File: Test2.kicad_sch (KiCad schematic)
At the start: 14 parts, among them J1 Raspberry_Pi_2_3, J1_GPIO4 01×06, J2_GPIO17 Conn_01x06_Socket, J3_GPIO27 Conn_01x06_Socket, J4_GPIO22 Conn_01x06_Socket, M1_GPIO23 Motor_Servo, SW1_GPIO8 SW_Push

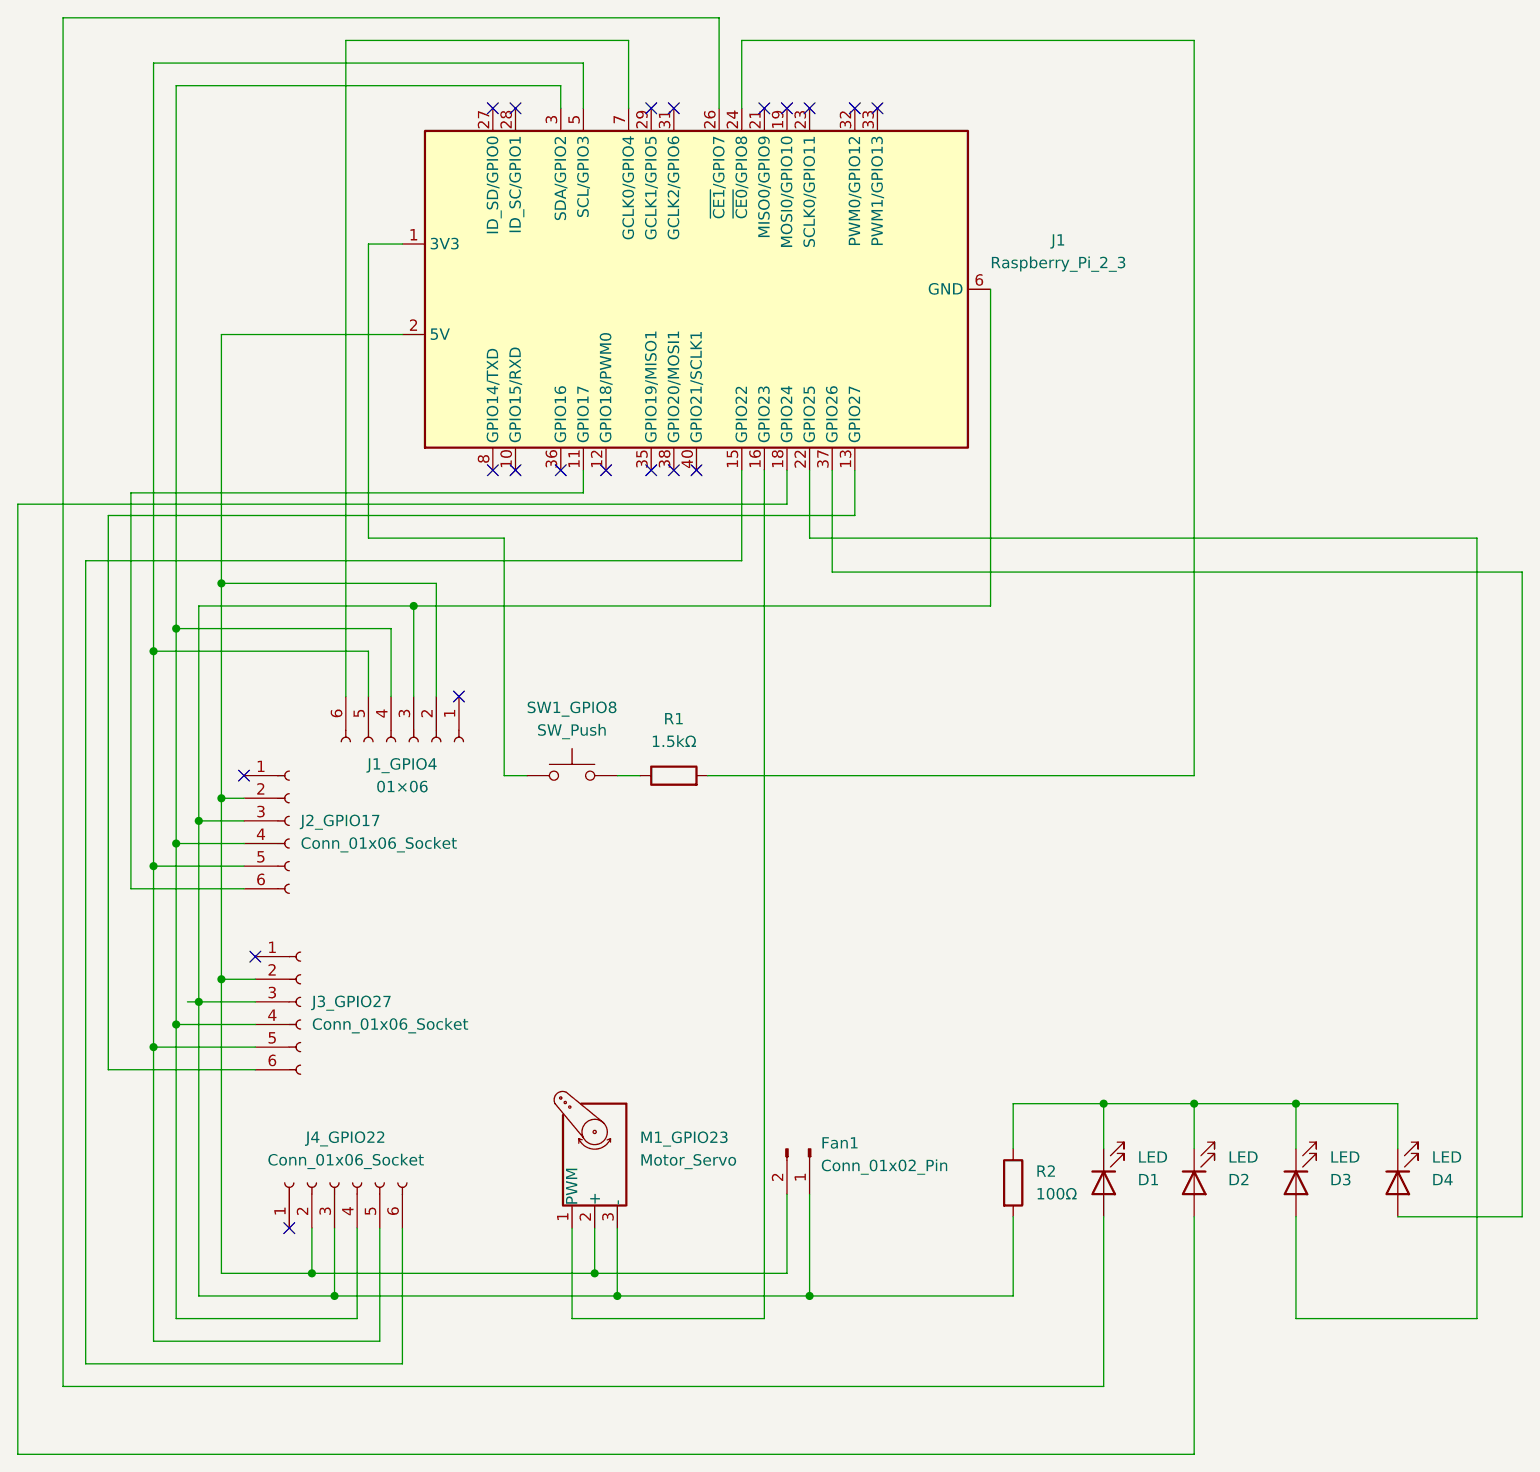
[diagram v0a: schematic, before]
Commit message: Initial commit
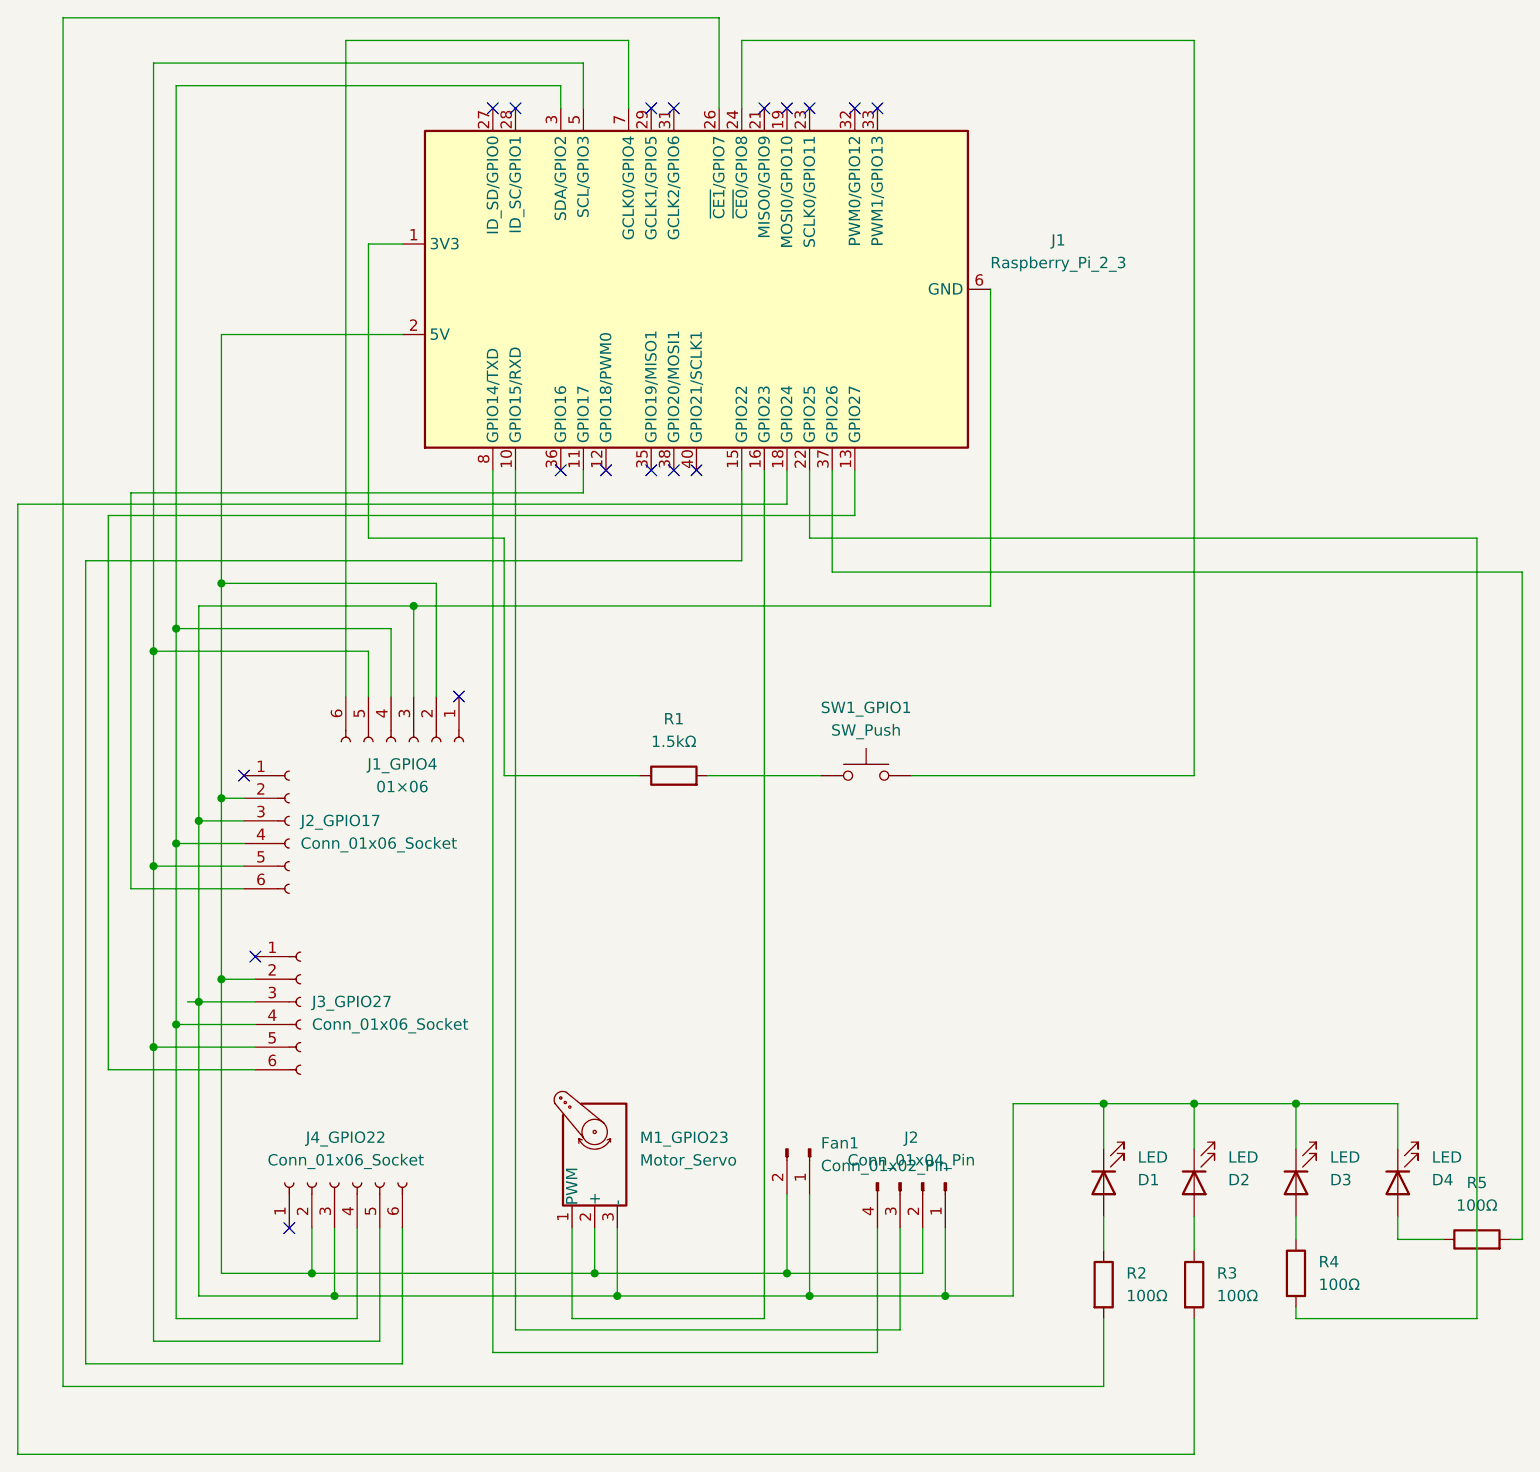
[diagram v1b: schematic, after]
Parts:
- removed SW1_GPIO8: SW_Push, ZHpretty:PushButton, symbol Switch:SW_Push
- added J2: Conn_01x04_Pin, Library:Grove_1x04, symbol Connector:Conn_01x04_Pin
- added R3, R4, R5: 100Ω, Resistor_SMD:R_0805_2012Metric, symbol Device:R
- added SW1_GPIO1: SW_Push, ZHpretty:PushButton, symbol Switch:SW_Push
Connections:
- net at Fan1.2 (Pin_2), J1.2 (5V), J1.4 (5V)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: now also J2.2 (Pin_2)
- net at Fan1.1 (Pin_1), J1.14 (GND), J1.20 (GND)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: now also D1.1 (K), D2.1 (K), D3.1 (K), D4.1 (K), J2.1 (Pin_1); no longer R2.2
- net at D2.2 (A): now also R3.1; no longer J1.18 (GPIO24)
- net at R1.1: now also J1.1 (3V3), J1.17 (3V3)
- net at R1.2: now also SW1_GPIO1.1; no longer J1.24 (~{CE0}/GPIO8)
- net at J1.10 (GPIO15/RXD): now also J2.3 (Pin_3)
- net at J1.22 (GPIO25): now also R4.2; no longer D3.2 (A)
- net at D1.2 (A): now also R2.1; no longer J1.26 (~{CE1}/GPIO7)
- net at D4.2 (A): now also R5.1; no longer J1.37 (GPIO26)
- net at J1.8 (GPIO14/TXD): now also J2.4 (Pin_4)
- new net: J1.26 (~{CE1}/GPIO7), R2.2
- new net: J1.24 (~{CE0}/GPIO8), SW1_GPIO1.3
- new net: J1.37 (GPIO26), R5.2
- new net: J1.18 (GPIO24), R3.2
- new net: D3.2 (A), R4.1
- no-connect marks 20 -> 18
